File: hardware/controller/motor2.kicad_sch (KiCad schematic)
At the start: 55 parts, among them J5 Conn_01x01, J6 Conn_01x01, J7 Conn_01x01, J8 Conn_02x03_Odd_Even, Q2 AOD66406, Q3 AOD66406, Q4 AOD66406, Q5 AOD66406, Q6 AOD66406, Q7 AOD66406, U10 LM2105D, U11 MCP6541, U12 LM2105D, U13 MCP6541, U8 LM2105D, U9 MCP6541

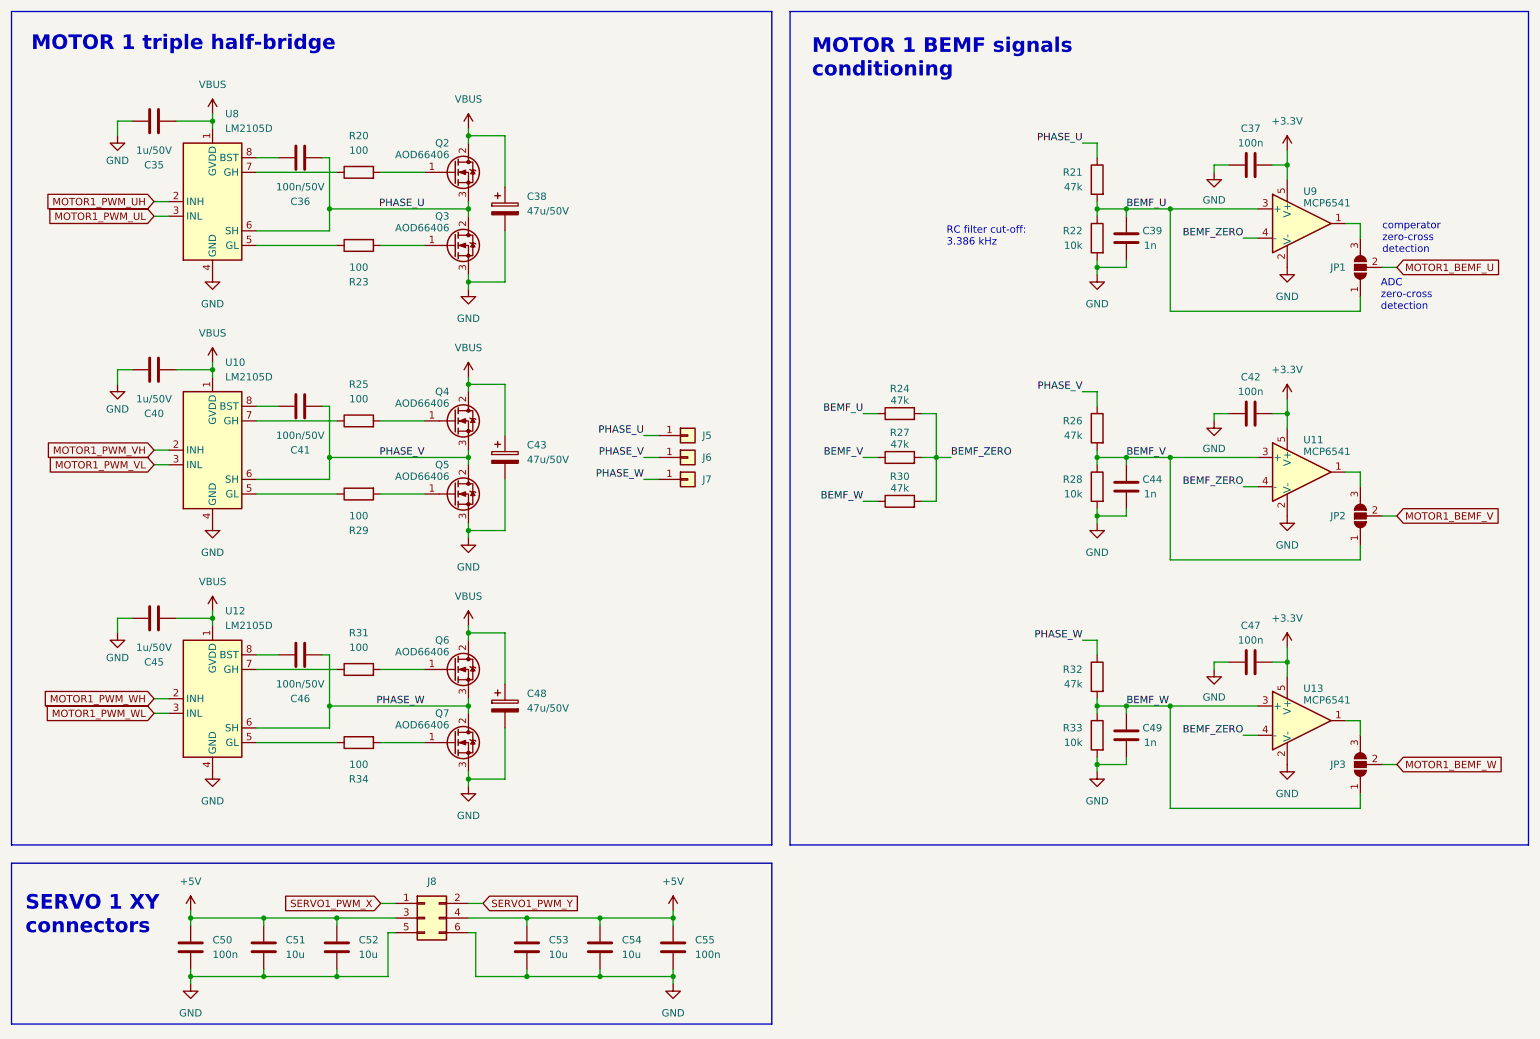
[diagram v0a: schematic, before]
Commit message: wip
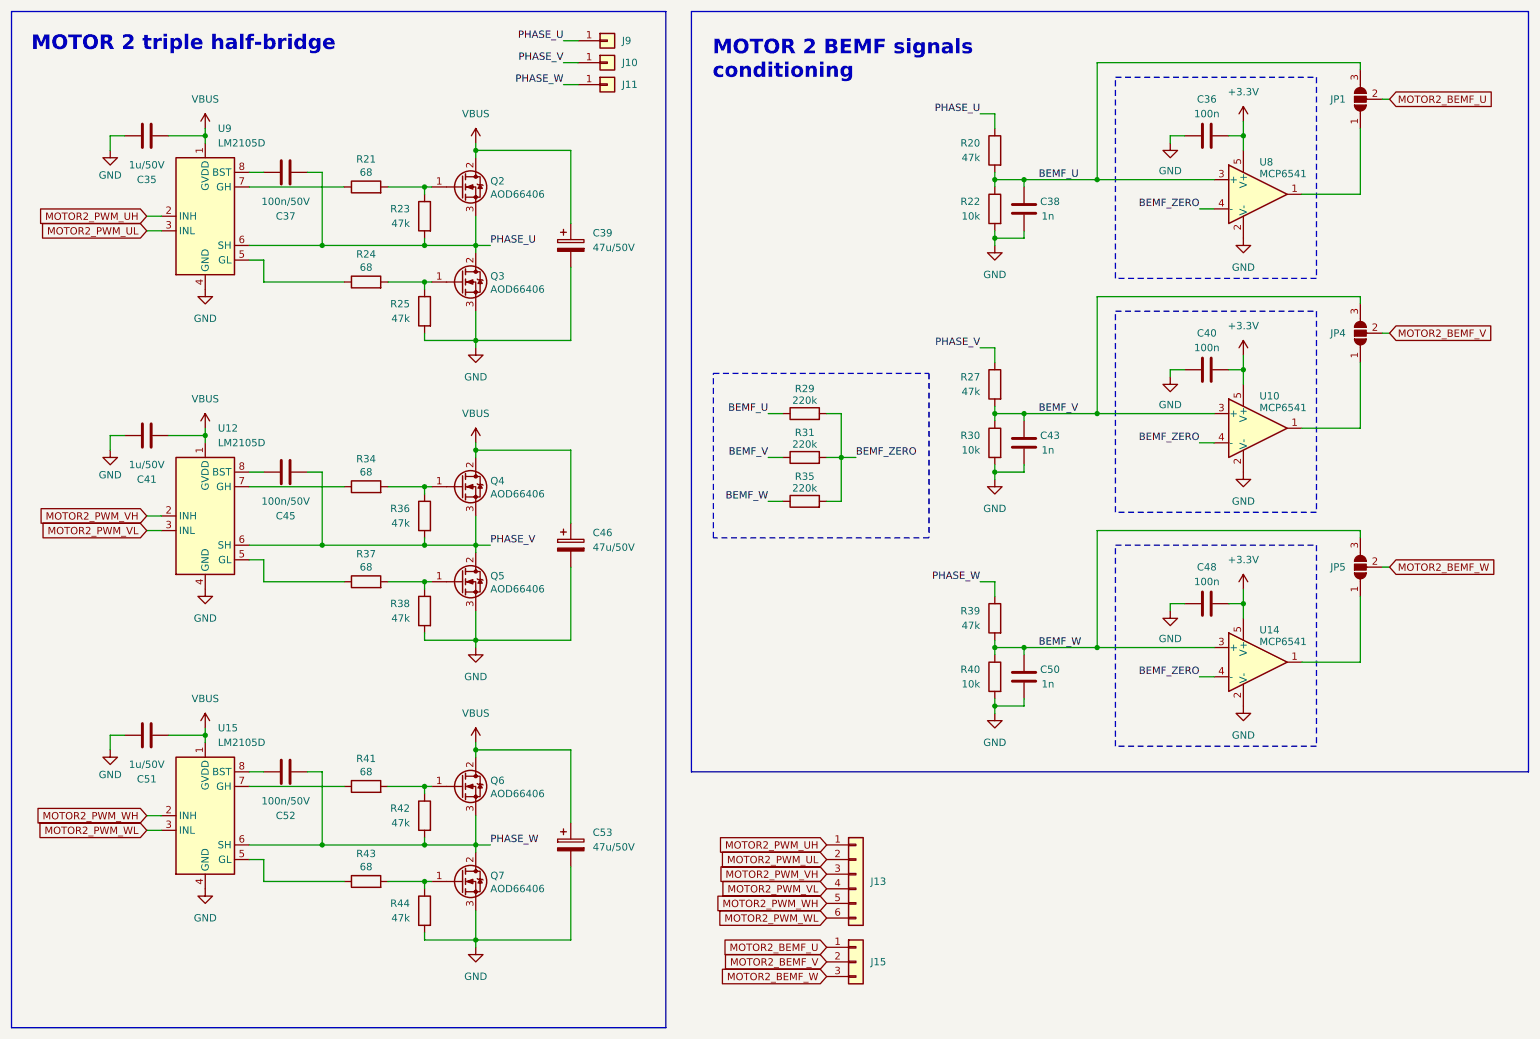
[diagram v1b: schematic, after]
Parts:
- removed C38, C43, C48: 47u/50V, Capacitor_SMD:CP_Elec_6.3x7.7, symbol Device:C_Polarized
- removed C39, C44, C49: 1n, Capacitor_SMD:C_0603_1608Metric, symbol Device:C
- removed C42, C47, C55: 100n, Capacitor_SMD:C_0603_1608Metric, symbol Device:C
- removed C46: 100n/50V, Capacitor_SMD:C_0603_1608Metric, symbol Device:C
- removed C53, C54: 10u, Capacitor_SMD:C_0603_1608Metric, symbol Device:C
- removed J5, J6, J7: Conn_01x01, Connector_Wire:SolderWire-2.5sqmm_1x01_D2.4mm_OD4.4mm, symbol Connector_Generic:Conn_01x01
- removed J8: Conn_02x03_Odd_Even, Connector_PinHeader_2.54mm:PinHeader_2x03_P2.54mm_Horizontal, symbol Connector_Generic:Conn_02x03_Odd_Even
- removed JP2, JP3: SolderJumper_3_Open, Jumper:SolderJumper-3_P1.3mm_Open_RoundedPad1.0x1.5mm, symbol Jumper:SolderJumper_3_Open
- removed R26, R32: 47k, Resistor_SMD:R_0603_1608Metric, symbol Device:R
- removed R28, R33: 10k, Resistor_SMD:R_0603_1608Metric, symbol Device:R
- removed U10, U8: LM2105D, Package_SO:SOIC-8_3.9x4.9mm_P1.27mm, symbol Driver_FET:LM2105D
- removed U11, U13, U9: MCP6541, Package_TO_SOT_SMD:SOT-23-5, symbol Comparator:MCP6561-OT
- added C38, C43: 1n, Capacitor_SMD:C_0603_1608Metric, symbol Device:C
- added C39, C46, C53: 47u/50V, Capacitor_SMD:CP_Elec_6.3x7.7, symbol Device:C_Polarized
- added C48: 100n, Capacitor_SMD:C_0603_1608Metric, symbol Device:C
- added J10, J11, J9: Conn_01x01, Connector_Wire:SolderWire-2.5sqmm_1x01_D2.4mm_OD4.4mm, symbol Connector_Generic:Conn_01x01
- added J13: Conn_01x06, symbol Connector_Generic:Conn_01x06
- added J15: Conn_01x03, symbol Connector_Generic:Conn_01x03
- added JP4, JP5: SolderJumper_3_Open, Jumper:SolderJumper-3_P1.3mm_Open_RoundedPad1.0x1.5mm, symbol Jumper:SolderJumper_3_Open
- added R35: 220k, Resistor_SMD:R_0603_1608Metric, symbol Device:R
- added R36, R38, R39, R42, R44: 47k, Resistor_SMD:R_0603_1608Metric, symbol Device:R
- added R37, R41, R43: 68, Resistor_SMD:R_0603_1608Metric, symbol Device:R
- added R40: 10k, Resistor_SMD:R_0603_1608Metric, symbol Device:R
- added U10, U14, U8: MCP6541, Package_TO_SOT_SMD:SOT-23-5, symbol Comparator:MCP6561-OT
- added U15, U9: LM2105D, Package_SO:SOIC-8_3.9x4.9mm_P1.27mm, symbol Driver_FET:LM2105D
- C36: value 100n/50V -> 100n
- C37: value 100n -> 100n/50V
- C40: value 1u/50V -> 100n
- C41: value 100n/50V -> 1u/50V
- C45: value 1u/50V -> 100n/50V
- C50: value 100n -> 1n
- C51: value 10u -> 1u/50V
- C52: value 10u -> 100n/50V
- R20, R23, R25: value 100 -> 47k
- R21, R24: value 47k -> 68
- R29, R31: value 100 -> 220k
- R30: value 47k -> 10k
- R34: value 100 -> 68
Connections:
- net +3.3V: now also C36.2, C40.2, C48.2, U10.5 (V+), U14.5 (V+), U8.5 (V+); no longer C37.2
- net BEMF_U: now also JP1.3 (B), R20.2, R29.1, C38.1, U8.3 (+); no longer JP1.1 (A), R21.2, R24.1
- net BEMF_V: now also R27.2, R30.1, R31.1, C43.1, JP4.3 (B), U10.3 (+); no longer R27.1
- net BEMF_W: now also C50.1, JP5.3 (B), R35.1, R39.2, R40.1, U14.3 (+); no longer R30.1
- net BEMF_ZERO: now also R29.2, R31.2, R35.2, U10.4 (-), U14.4 (-), U8.4 (-); no longer R24.2, R27.2, R30.2
- net GND: now also C36.1, C41.1, C51.1, R25.2, R30.2, C38.2, C39.2, C43.2, C46.2, C48.1, C53.2, R38.2, R40.2, R44.2, U10.2 (V-), U14.2 (V-), U15.4 (GND), U8.2 (V-), U9.4 (GND); no longer C37.1, C45.1, C51.2, C52.2
- net PHASE_U: now also C37.2, R20.1, R23.2, J9.1 (Pin_1), U9.6 (SH); no longer C36.2, R21.1
- net PHASE_V: now also C45.2, R27.1, U12.6 (SH), J10.1 (Pin_1), R36.2; no longer C41.2
- net PHASE_W: now also C52.2, J11.1 (Pin_1), R39.1, R42.2, U15.6 (SH); no longer U12.6 (SH)
- net VBUS: now also C41.2, C51.2, C39.1, C46.1, C53.1, U15.1 (GVDD), U9.1 (GVDD); no longer C40.2, C45.2
- net at Q5.1 (G): now also R37.2, R38.1; no longer R29.2
- net at U12.8 (BST): now also C45.1
- net at U12.5 (GL): now also R37.1; no longer R34.1
- net at U12.7 (GH): now also R34.1; no longer R31.1
- net at Q6.1 (G): now also R41.2, R42.1; no longer R31.2
- net at Q2.1 (G): now also R21.2, R23.1; no longer R20.2
- net at Q3.1 (G): now also R24.2, R25.1; no longer R23.2
- net at Q4.1 (G): now also R34.2, R36.1; no longer R25.2
- net at Q7.1 (G): now also R43.2, R44.1; no longer R34.2
- removed net +5V: C50.1, C51.1, C52.1
- net MOTOR1_BEMF_U renamed MOTOR2_BEMF_U
- net MOTOR2_BEMF_U: now also J15.1 (Pin_1)
- net MOTOR1_PWM_WH renamed MOTOR2_PWM_VH
- net MOTOR2_PWM_VH: now also J13.3 (Pin_3)
- net MOTOR1_PWM_WL renamed MOTOR2_PWM_VL
- net MOTOR2_PWM_VL: now also J13.4 (Pin_4)
- new net: JP1.1 (A), U8.1
- new net: R21.1, U9.7 (GH)
- new net: JP5.1 (A), U14.1
- new net: JP4.1 (A), U10.1
- new net: R24.1, U9.5 (GL)
- new net: C37.1, U9.8 (BST)
- new net: R43.1, U15.5 (GL)
- new net: R41.1, U15.7 (GH)
- new net: C52.1, U15.8 (BST)
- new net MOTOR2_BEMF_V: J15.2 (Pin_2), JP4.2 (C)
- new net MOTOR2_BEMF_W: J15.3 (Pin_3), JP5.2 (C)
- new net MOTOR2_PWM_UH: J13.1 (Pin_1), U9.2 (INH)
- new net MOTOR2_PWM_UL: J13.2 (Pin_2), U9.3 (INL)
- new net MOTOR2_PWM_WH: J13.5 (Pin_5), U15.2 (INH)
- new net MOTOR2_PWM_WL: J13.6 (Pin_6), U15.3 (INL)
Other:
- note added: "MOTOR 2 BEMF signals conditioning"
- note added: "MOTOR 2 triple half-bridge"
- note removed: "ADC zero-cross detection"
- note removed: "MOTOR 1 BEMF signals conditioning"
- note removed: "MOTOR 1 triple half-bridge"
- note removed: "RC filter cut-off: 3.386 kHz"
- note removed: "SERVO 1 XY connectors"
- note removed: "comperator zero-cross detection"
